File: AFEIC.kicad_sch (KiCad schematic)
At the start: 31 parts, among them J1 CONN HEADER VERT 6POS 1.5MM, U1 TLE9012DQUXUMA1

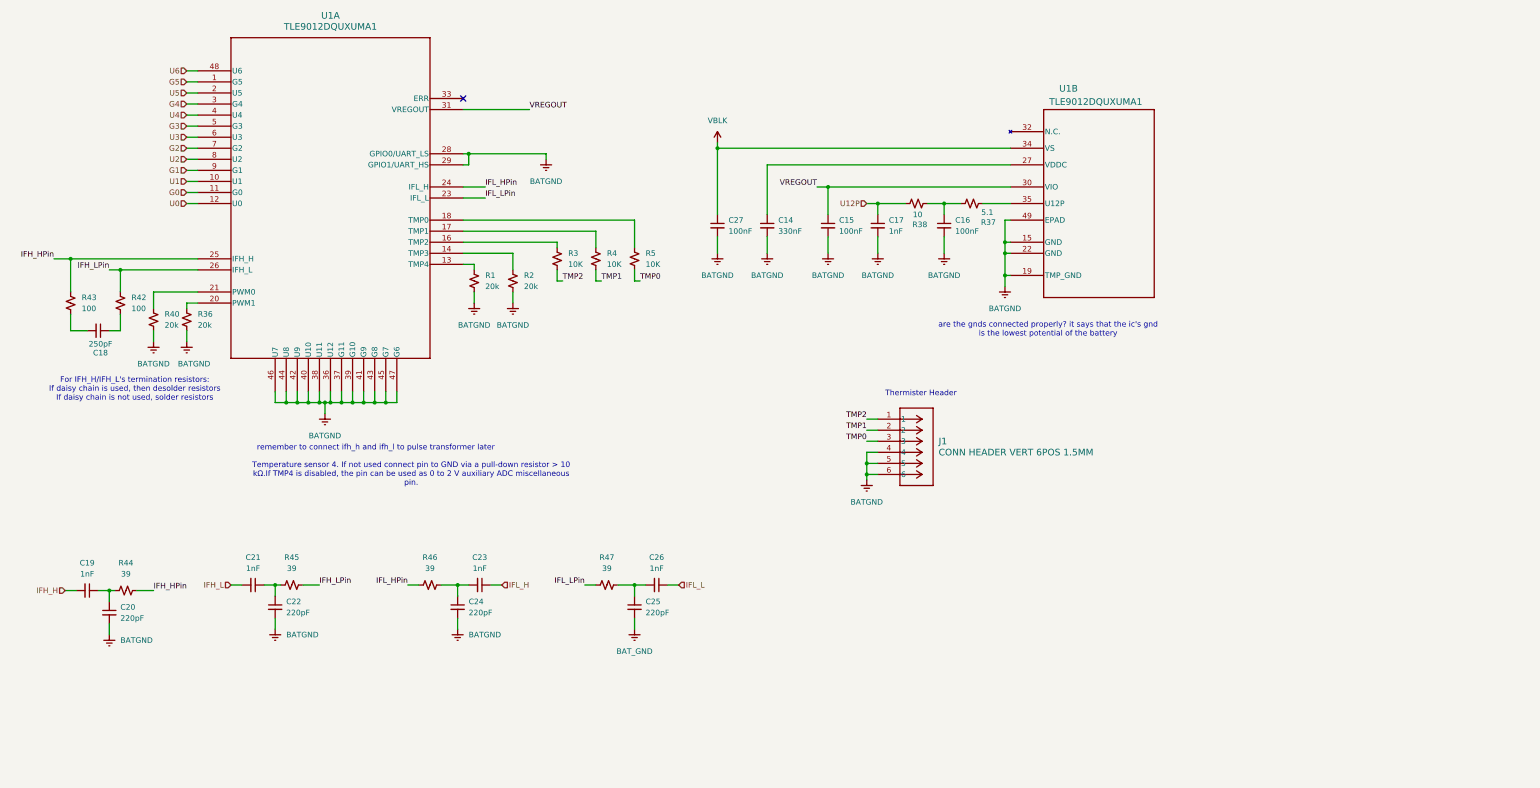
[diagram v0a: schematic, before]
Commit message: finished schematic
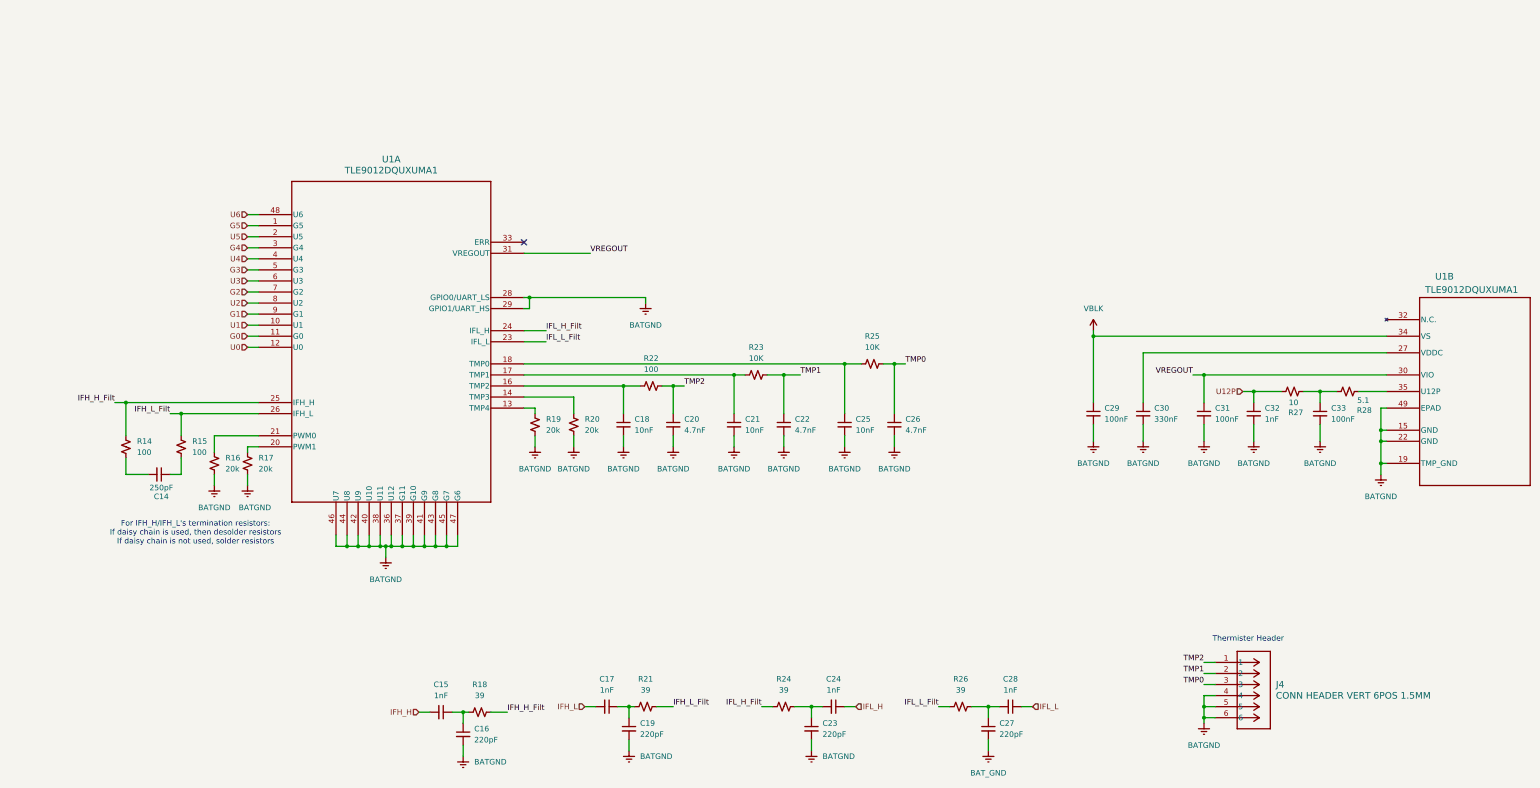
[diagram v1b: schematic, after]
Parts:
- removed R3, R4, R5: 10K, symbol Device:R_Small_US
- added C18, C21, C25: 10nF, symbol Device:C_Small
- added C20, C22, C26: 4.7nF, symbol Device:C_Small
- added R22: 100, symbol Device:R_Small_US
- added R23, R25: 10K, symbol Device:R_Small_US
- renumbered C18 to C14, C19 to C15, C20 to C16, C21 to C17, C22 to C19, C24 to C23, C23 to C24, C25 to C27, C26 to C28, C27 to C29, C14 to C30, C15 to C31, C17 to C32, C16 to C33, J1 to J4, R43 to R14, R42 to R15, R40 to R16, R36 to R17, R44 to R18, R1 to R19, R2 to R20, R45 to R21, R46 to R24, R47 to R26, R38 to R27, R37 to R28
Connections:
- net BATGND: now also C18.2, C20.2, C21.2, C22.2, C25.2, C26.2
- net TMP0: now also C26.1, R25.2
- net TMP1: now also C22.1, R23.2
- net TMP2: now also C20.1, R22.2
- net at U1.17 (TMP1): now also C21.1, R23.1
- net at U1.16 (TMP2): now also C18.1, R22.1
- net at U1.18 (TMP0): now also C25.1, R25.1
- net IFH_HPin renamed IFH_H_Filt
- net IFH_LPin renamed IFH_L_Filt
- net IFL_HPin renamed IFL_H_Filt
- net IFL_LPin renamed IFL_L_Filt
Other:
- note removed: "Temperature sensor 4. If not used connect pin to GND via a pull-down resistor > 10 kΩ.If TMP4 is disabled, the pin can be used as 0 to 2 V auxiliary ADC miscellaneous pin."
- note removed: "are the gnds connected properly? it says that the ic's gnd is the lowest potential of the battery"
- note removed: "remember to connect ifh_h and ifh_l to pulse transformer later"
- moved on the sheet: C14, C15, C16, C17, C19, C23, C24, C27, C28, C29, C30, C31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

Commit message: passive values
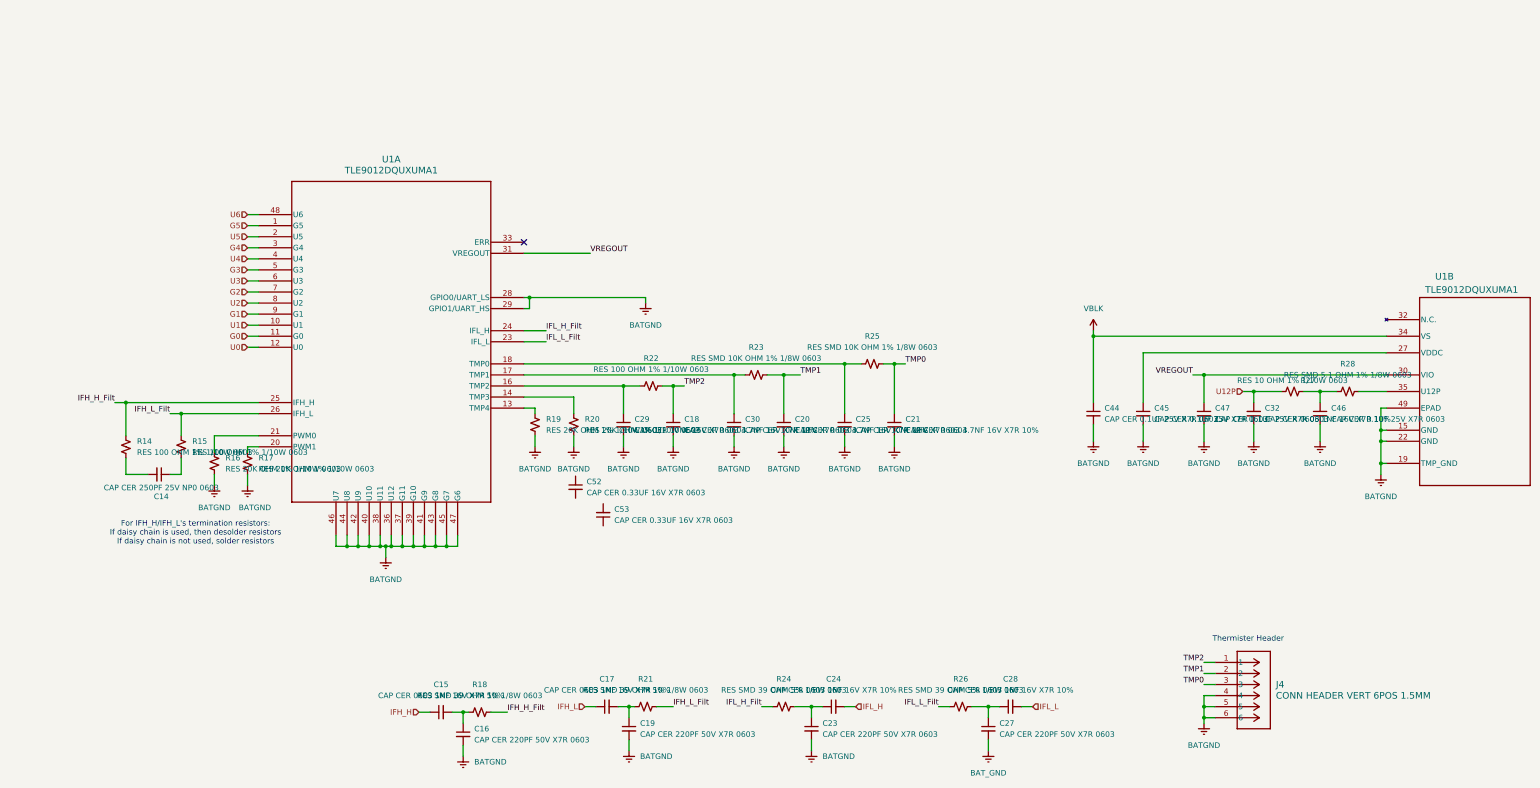
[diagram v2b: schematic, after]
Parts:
- removed C22, C26: 4.7nF, symbol Device:C_Small
- removed C31, C33: 100nF, symbol Device:C_Small
- added C44, C45, C46, C47: CAP CER 0.1UF 25V X7R 0603, Capacitor_SMD:C_0603_1608Metric, symbol Device:C_Small
- added C52, C53: CAP CER 0.33UF 16V X7R 0603, Capacitor_SMD:C_0603_1608Metric, symbol Device:C_Small
- C14: value 250pF -> CAP CER 250PF 25V NP0 0603; footprint (none) -> Capacitor_SMD:C_0603_1608Metric
- C15, C17, C24, C28, C32: value 1nF -> CAP CER 0603 1NF 16V X7R 10%; footprint (none) -> Capacitor_SMD:C_0603_1608Metric
- C16, C19, C23, C27: value 220pF -> CAP CER 220PF 50V X7R 0603; footprint (none) -> Capacitor_SMD:C_0603_1608Metric
- C18, C21: value 10nF -> CAP CER 0603 4.7NF 16V X7R 10%; footprint (none) -> Capacitor_SMD:C_0603_1608Metric
- C20: value 4.7nF -> CAP CER 0603 4.7NF 16V X7R 10%; footprint (none) -> Capacitor_SMD:C_0603_1608Metric
- C25: value 10nF -> CAP CER 10NF 16V X7R 0603; footprint (none) -> Capacitor_SMD:C_0603_1608Metric
- C29: value 100nF -> CAP CER 10NF 16V X7R 0603; footprint (none) -> Capacitor_SMD:C_0603_1608Metric
- C30: value 330nF -> CAP CER 10NF 16V X7R 0603; footprint (none) -> Capacitor_SMD:C_0603_1608Metric
- R14, R15, R22: value 100 -> RES 100 OHM 1% 1/10W 0603; footprint (none) -> Resistor_SMD:R_0603_1608Metric
- R16, R17, R19, R20: value 20k -> RES 20K OHM 1% 1/10W 0603; footprint (none) -> Capacitor_SMD:C_0603_1608Metric
- R18, R21, R24, R26: value 39 -> RES SMD 39 OHM 5% 1/8W 0603; footprint (none) -> Resistor_SMD:R_0603_1608Metric; LCSC (none) -> C2079967
- R23, R25: value 10K -> RES SMD 10K OHM 1% 1/8W 0603; footprint (none) -> Resistor_SMD:R_0603_1608Metric; LCSC (none) -> C844918
- R27: value 10 -> RES 10 OHM 1% 1/10W 0603; footprint (none) -> Resistor_SMD:R_0603_1608Metric
- R28: value 5.1 -> RES SMD 5.1 OHM 1% 1/8W 0603; footprint (none) -> Resistor_SMD:R_0603_1608Metric; LCSC (none) -> C242492
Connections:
- net BATGND: now also C32.1, C44.2, C45.2, C46.2, C47.2; no longer C32.2
- net IFH_H: now also C15.1; no longer C15.2
- net IFH_H_Filt: now also R14.2; no longer R14.1
- net IFH_L: now also C17.1; no longer C17.2
- net IFH_L_Filt: now also R15.2; no longer R15.1
- net IFL_H: now also C24.2; no longer C24.1
- net IFL_L: now also C28.2; no longer C28.1
- net TMP0: now also C21.1
- net TMP1: now also C20.1
- net TMP2: now also C18.1; no longer C20.1
- net U12P: now also C32.2; no longer C32.1
- net VBLK: now also C44.1; no longer C29.1
- net VREGOUT: now also C47.1
- net at R23.1, U1.17 (TMP1): now also C30.1; no longer C21.1
- net at C16.1, R18.1: now also C15.2; no longer C15.1
- net at C23.1, R24.2: now also C24.1; no longer C24.2
- net at C27.1, R26.2: now also C28.1; no longer C28.2
- net at C19.1, R21.1: now also C17.2; no longer C17.1
- net at U1.27 (VDDC): now also C45.1; no longer C30.1
- net at R27.2, R28.1: now also C46.1
- net at C14.2: now also R14.1; no longer R14.2
- net at C14.1: now also R15.1; no longer R15.2
- net at R22.1, U1.16 (TMP2): now also C29.1; no longer C18.1
